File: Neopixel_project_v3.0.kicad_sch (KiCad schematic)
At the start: 64 parts, among them J1 Conn_01x03_Pin, J2 Conn_01x02_Pin, Q1 MMBT3904, Q2 MMBT3904, Q3 MMBT3904, Q4 MMBT3904, Q5 DO3407B, Q6 DO3407B, Q7 DO3407B, Q8 DO3407B, SW1 TS-1088-AR02016, SW2 TS-1088-AR02016, U1 ESP8685H4, U2 AL8843, U3 TD1469, U4 USBLC6-4SC6, Y1 Crystal_GND24

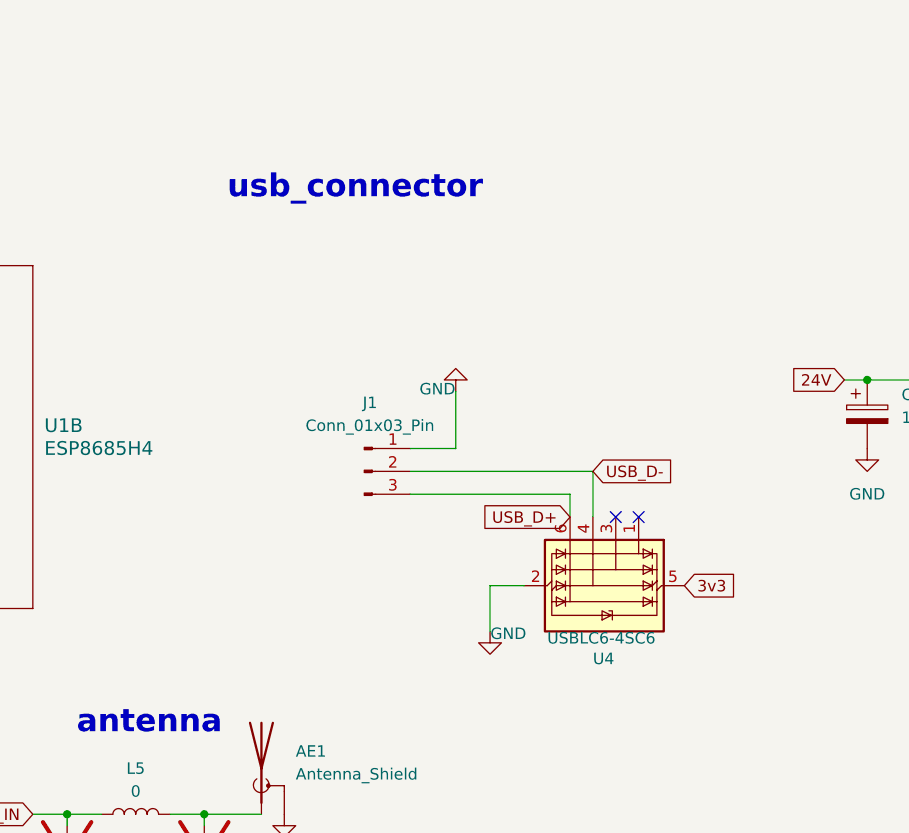
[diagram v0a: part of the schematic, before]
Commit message: pcb finished
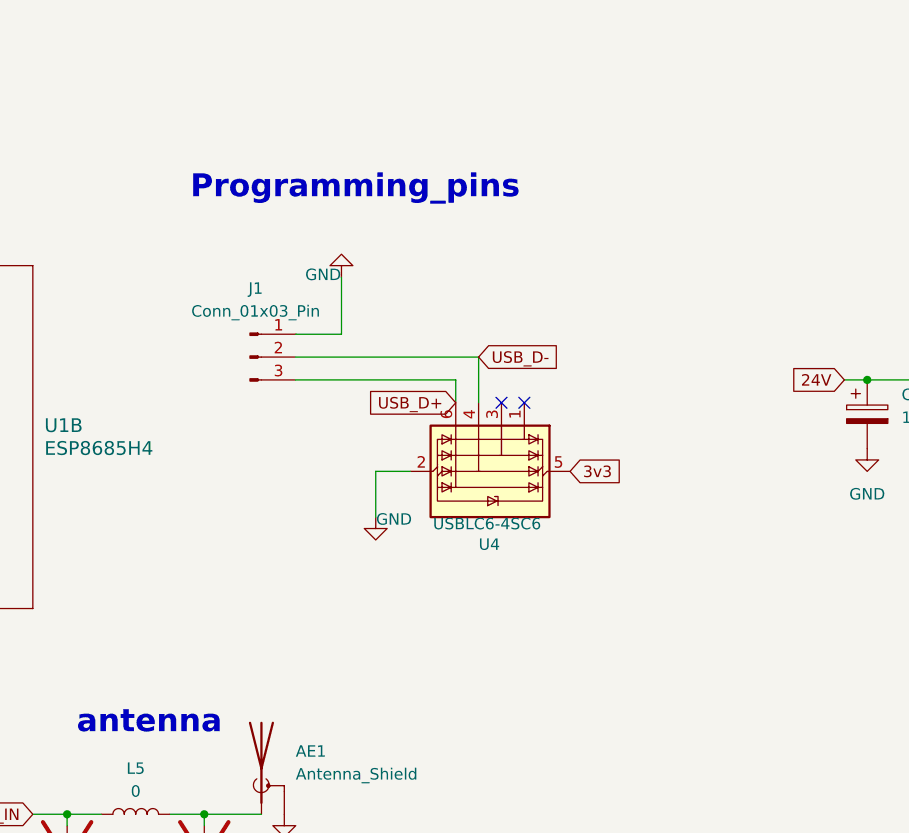
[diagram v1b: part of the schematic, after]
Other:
- note added: "Programming_pins"
- note removed: "usb_connector"
- moved on the sheet: J1, U4
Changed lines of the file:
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@@
 	)
 	(no_connect
-		(at 172.72 53.34)
+		(at 160.02 40.64)
 	)
 	(no_connect
@@
 	)
 	(no_connect
-		(at 175.26 53.34)
+		(at 162.56 40.64)
 	)
 	(no_connect
@@
 	(wire
 		(pts
-			(xy 149.86 50.8) (xy 167.64 50.8)
+			(xy 137.16 38.1) (xy 154.94 38.1)
 		)
 		(stroke
@@
 	(wire
 		(pts
-			(xy 158.75 60.96) (xy 162.56 60.96)
+			(xy 146.05 48.26) (xy 149.86 48.26)
 		)
 		(stroke
@@
 	(wire
 		(pts
-			(xy 149.86 48.26) (xy 170.18 48.26)
+			(xy 137.16 35.56) (xy 157.48 35.56)
 		)
 		(stroke
@@
 	(wire
 		(pts
-			(xy 154.94 45.72) (xy 154.94 39.37)
+			(xy 142.24 33.02) (xy 142.24 26.67)
 		)
 		(stroke
@@
 	(wire
 		(pts
-			(xy 167.64 50.8) (xy 167.64 53.34)
+			(xy 154.94 38.1) (xy 154.94 40.64)
 		)
 		(stroke
@@
 	(wire
 		(pts
-			(xy 158.75 66.04) (xy 158.75 60.96)
+			(xy 146.05 53.34) (xy 146.05 48.26)
 		)
 		(stroke
@@
 	(wire
 		(pts
-			(xy 170.18 48.26) (xy 170.18 53.34)
+			(xy 157.48 35.56) (xy 157.48 40.64)
 		)
 		(stroke
@@
 	(wire
 		(pts
-			(xy 149.86 45.72) (xy 154.94 45.72)
+			(xy 137.16 33.02) (xy 142.24 33.02)
 		)
 		(stroke
@@
 		)
 	)
-	(text "usb_connector"
+	(text "Programming_pins"
 		(exclude_from_sim no)
 		(at 143.764 16.764 0)
@@
 	(global_label "USB_D+"
 		(shape input)
-		(at 167.64 53.34 180)
+		(at 154.94 40.64 180)
 		(fields_autoplaced yes)
 		(effects
@@
 		)
 		(property "Intersheetrefs" "${INTERSHEET_REFS}"
-			(at 157.0348 53.34 0)
+			(at 144.3348 40.64 0)
 			(effects
 				(font
@@
 	(global_label "3v3"
 		(shape input)
-		(at 180.34 60.96 0)
+		(at 167.64 48.26 0)
 		(fields_autoplaced yes)
 		(effects
@@
 		)
 		(property "Intersheetrefs" "${INTERSHEET_REFS}"
-			(at 186.7118 60.96 0)
+			(at 174.0118 48.26 0)
 			(effects
 				(font
@@
 	(global_label "USB_D-"
 		(shape input)
-		(at 170.18 48.26 0)
+		(at 157.48 35.56 0)
 		(fields_autoplaced yes)
 		(effects
@@
 		)
 		(property "Intersheetrefs" "${INTERSHEET_REFS}"
-			(at 180.7852 48.26 0)
+			(at 168.0852 35.56 0)
 			(effects
 				(font
@@
 	(symbol
 		(lib_id "Connector:Conn_01x03_Pin")
-		(at 144.78 48.26 0)
+		(at 132.08 35.56 0)
 		(unit 1)
 		(exclude_from_sim no)
@@
 		(fields_autoplaced yes)
 		(property "Reference" "J1"
-			(at 145.415 40.64 0)
+			(at 132.715 27.94 0)
 			(effects
 				(font
@@
 		)
 		(property "Value" "Conn_01x03_Pin"
-			(at 145.415 43.18 0)
+			(at 132.715 30.48 0)
 			(effects
 				(font
@@
 		)
 		(property "Footprint" "Connector_PinHeader_2.54mm:PinHeader_1x03_P2.54mm_Vertical"
-			(at 144.78 48.26 0)
+			(at 132.08 35.56 0)
 			(effects
 				(font
@@
 		)
 		(property "Datasheet" "~"
-			(at 144.78 48.26 0)
+			(at 132.08 35.56 0)
 			(effects
 				(font
@@
 		)
 		(property "Description" "Generic connector, single row, 01x03, script generated"
-			(at 144.78 48.26 0)
+			(at 132.08 35.56 0)
 			(effects
 				(font
@@
 	(symbol
 		(lib_id "power:GND")
-		(at 158.75 66.04 0)
+		(at 146.05 53.34 0)
 		(unit 1)
 		(exclude_from_sim no)
@@
 		(dnp no)
 		(property "Reference" "#PWR026"
-			(at 158.75 72.39 0)
+			(at 146.05 59.69 0)
 			(effects
 				(font
@@
 		)
 		(property "Value" "GND"
-			(at 160.782 66.294 0)
+			(at 148.082 53.594 0)
 			(effects
 				(font
@@
 		)
 		(property "Footprint" ""
-			(at 158.75 66.04 0)
+			(at 146.05 53.34 0)
 			(effects
 				(font
@@
 		)
 		(property "Datasheet" ""
-			(at 158.75 66.04 0)
+			(at 146.05 53.34 0)
 			(effects
 				(font
@@
 		)
 		(property "Description" "Power symbol creates a global label with name \"GND\" , ground"
-			(at 158.75 66.04 0)
+			(at 146.05 53.34 0)
 			(effects
 				(font
@@
 	(symbol
 		(lib_id "Power_Protection:USBLC6-4SC6")
-		(at 172.72 60.96 270)
+		(at 160.02 48.26 270)
 		(unit 1)
 		(exclude_from_sim no)
@@
 		(dnp no)
 		(property "Reference" "U4"
-			(at 170.18 69.088 90)
+			(at 157.48 56.388 90)
 			(effects
 				(font
@@
 		)
 		(property "Value" "USBLC6-4SC6"
-			(at 165.1 66.802 90)
+			(at 152.4 54.102 90)
 			(effects
 				(font
@@
 		)
 		(property "Footprint" "Package_TO_SOT_SMD:SOT-23-6"
-			(at 162.56 63.5 0)
+			(at 149.86 50.8 0)
 			(effects
 				(font
@@
 		)
 		(property "Datasheet" "https://www.st.com/resource/en/datasheet/usblc6-4.pdf"
-			(at 160.02 63.5 0)
+			(at 147.32 50.8 0)
 			(effects
 				(font
@@
 		)
 		(property "Description" "Very low capacitance ESD protection diode, 4 data-line, SOT-23-6"
-			(at 172.72 60.96 0)
+			(at 160.02 48.26 0)
 			(effects
 				(font
@@
 	(symbol
 		(lib_id "power:GND")
-		(at 154.94 39.37 180)
+		(at 142.24 26.67 180)
 		(unit 1)
 		(exclude_from_sim no)
@@
 		(dnp no)
 		(property "Reference" "#PWR020"
-			(at 154.94 33.02 0)
+			(at 142.24 20.32 0)
 			(effects
 				(font
@@
 		)
 		(property "Value" "GND"
-			(at 152.908 39.116 0)
+			(at 140.208 26.416 0)
 			(effects
 				(font
@@
 		)
 		(property "Footprint" ""
-			(at 154.94 39.37 0)
+			(at 142.24 26.67 0)
 			(effects
 				(font
@@
 		)
 		(property "Datasheet" ""
-			(at 154.94 39.37 0)
+			(at 142.24 26.67 0)
 			(effects
 				(font
@@
 		)
 		(property "Description" "Power symbol creates a global label with name \"GND\" , ground"
-			(at 154.94 39.37 0)
+			(at 142.24 26.67 0)
 			(effects
 				(font
